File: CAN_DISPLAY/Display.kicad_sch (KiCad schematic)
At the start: 14 parts, among them J1 DISPLAY, J14 Display, J2 I2C Sensor 1, J3 I2C Sensor 2, U6 BME280

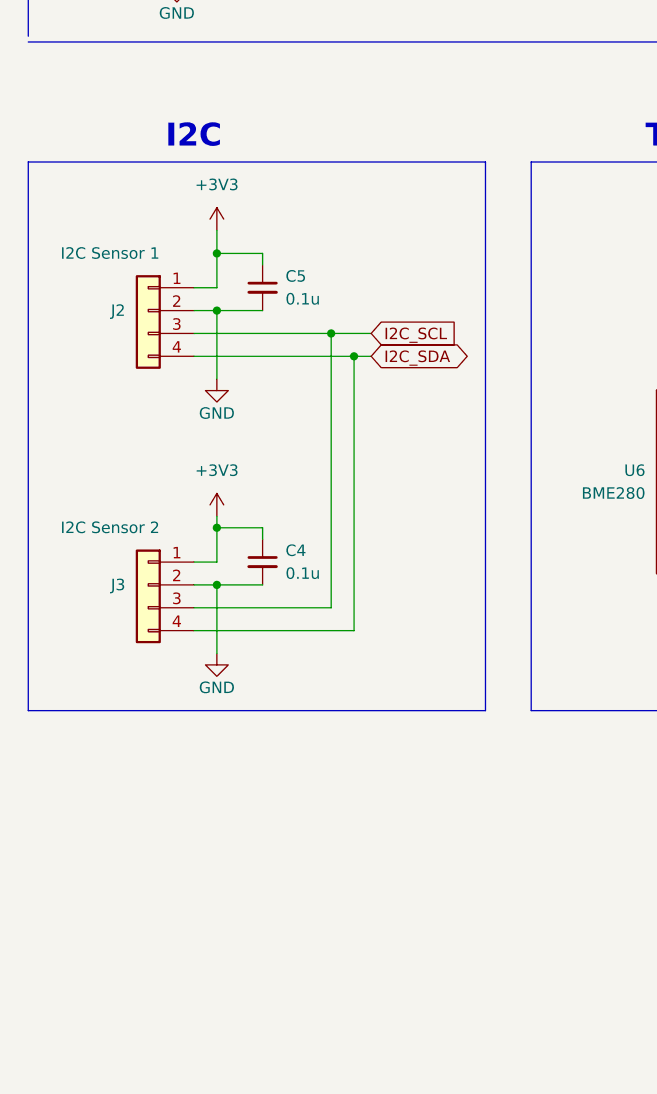
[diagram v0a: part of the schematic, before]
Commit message: PCB Fixes
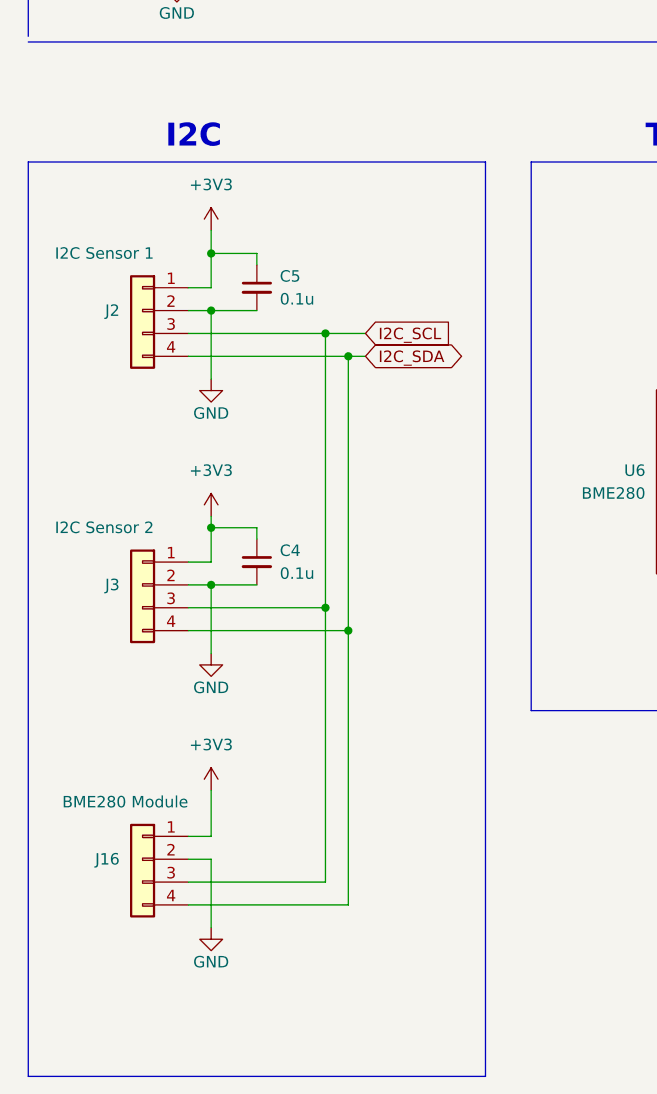
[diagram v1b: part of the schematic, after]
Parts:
- added J16: BME280 Module, Connector_PinHeader_2.54mm:PinHeader_1x04_P2.54mm_Vertical, symbol Connector_Generic:Conn_01x04
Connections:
- net +3V3: now also J16.1 (Pin_1)
- net GND: now also J16.2 (Pin_2)
- net I2C_SCL: now also J16.3 (Pin_3)
- net I2C_SDA: now also J16.4 (Pin_4)
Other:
- moved on the sheet: C4, C5, J2, J3
